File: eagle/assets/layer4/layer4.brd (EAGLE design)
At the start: 102.9 x 102.9 mm, 45 parts, among them Y1 8MHz

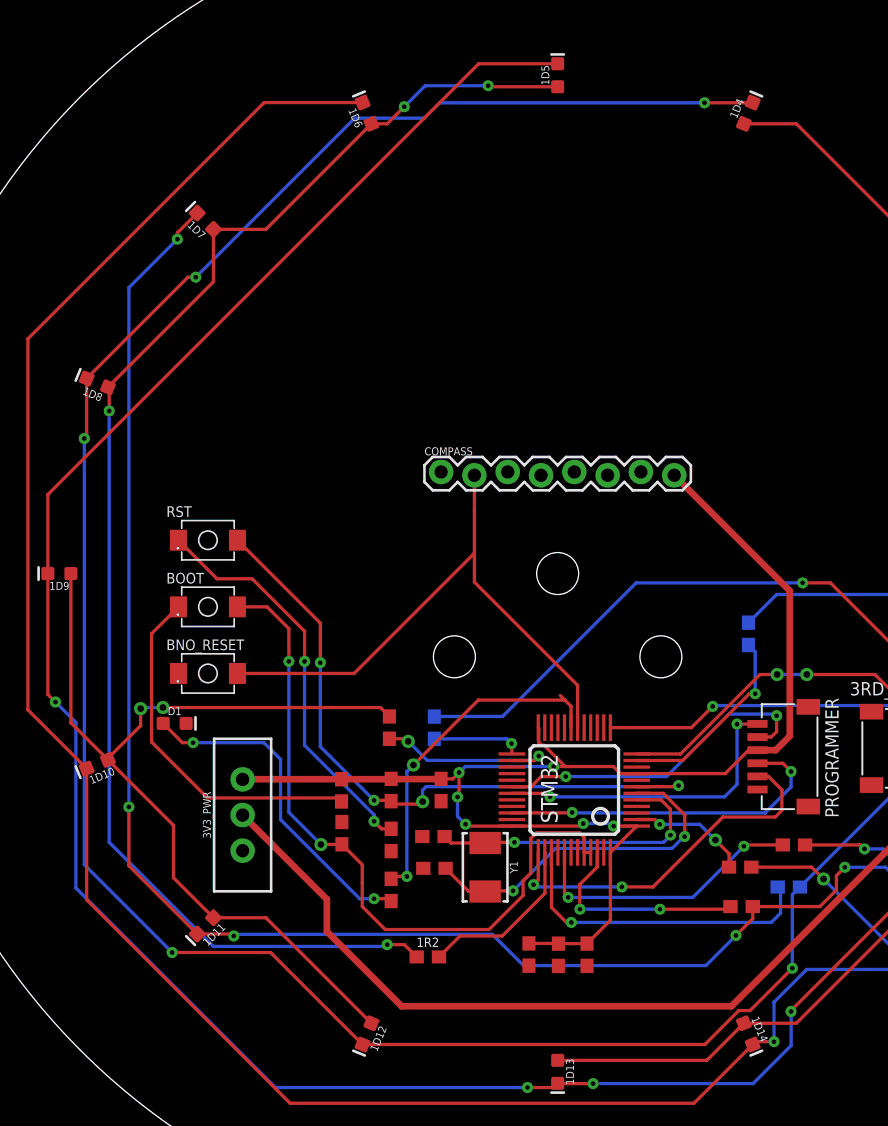
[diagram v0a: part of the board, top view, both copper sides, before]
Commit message: more shit need to do
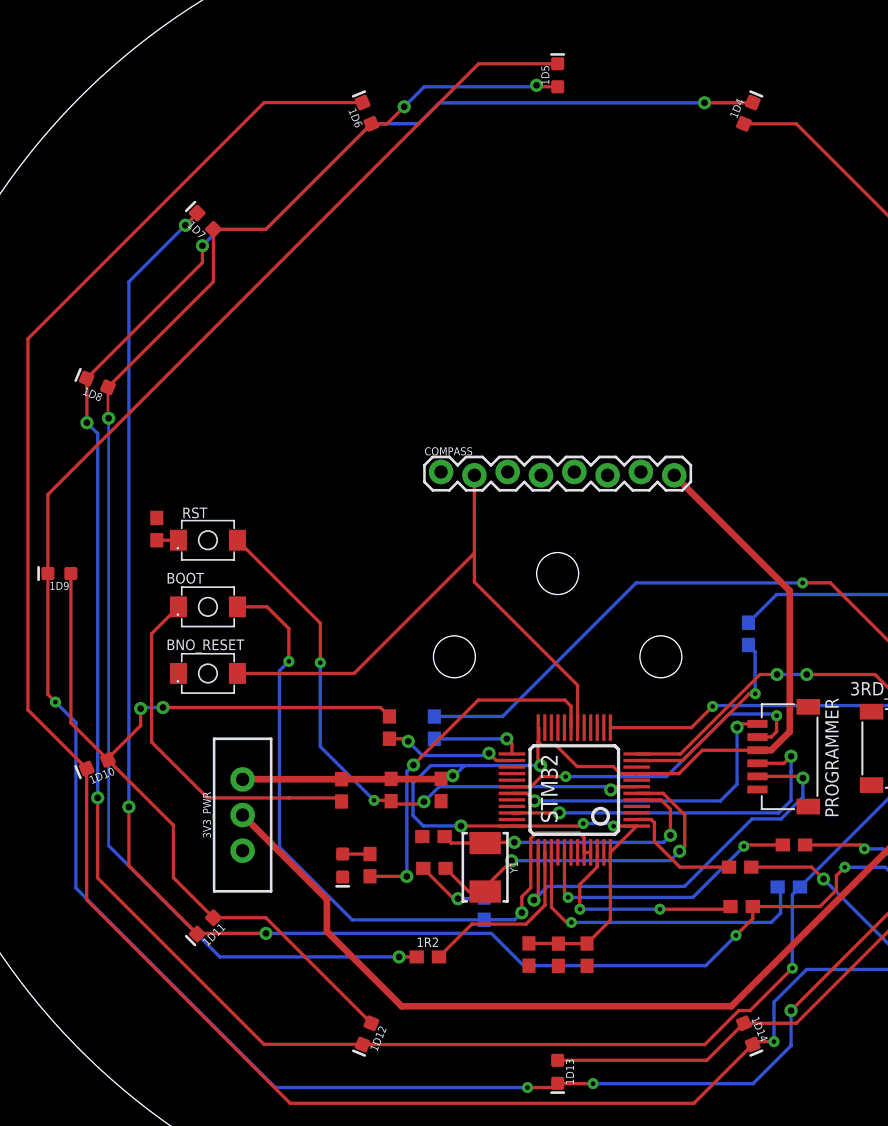
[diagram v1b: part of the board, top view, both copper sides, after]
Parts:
- moved R2 29.7 mm to (-30.6, 3.39), turned to 270 degrees
- moved D1 16.8 mm to (-16.4, -22.3), turned to 270 degrees
- moved R4 12.3 mm to (-5.60, -25.6), flipped to the bottom
- moved R5 2.48 mm to (-14.3, -22.2), turned to 270 degrees
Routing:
- net N$70: track 30.7 -> 1.65 mm, vias 2 -> 0
- net N$74: track 25.7 -> 2.08 mm, vias 2 -> 0
- net 3V3_SWITCH: track 103.5 -> 110.5 mm, vias 6 -> 5
- net RESET: track 51.9 -> 45.1 mm
- net GND: track 0.00 -> 5.65 mm, vias 0 -> 1
- net SWCLK: track 27.9 -> 32.5 mm
- net L3R: track 14.4 -> 10.2 mm
- net SWDIO: track 26.1 -> 27.8 mm
- net N$73: track 26.4 -> 27.4 mm
- net BOOT0: track 53.8 -> 54.6 mm
- net OSC_OUT: track 26.7 -> 27.4 mm
- net N$24: track 186.9 -> 187.5 mm
- net L2R: track 13.2 -> 13.7 mm
- net L2C: track 9.15 -> 9.39 mm, vias 2 -> 0
